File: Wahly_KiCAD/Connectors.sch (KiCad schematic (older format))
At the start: 9 parts, among them J2 Power, J3 ADC, J4 SWD, J5 TIM2

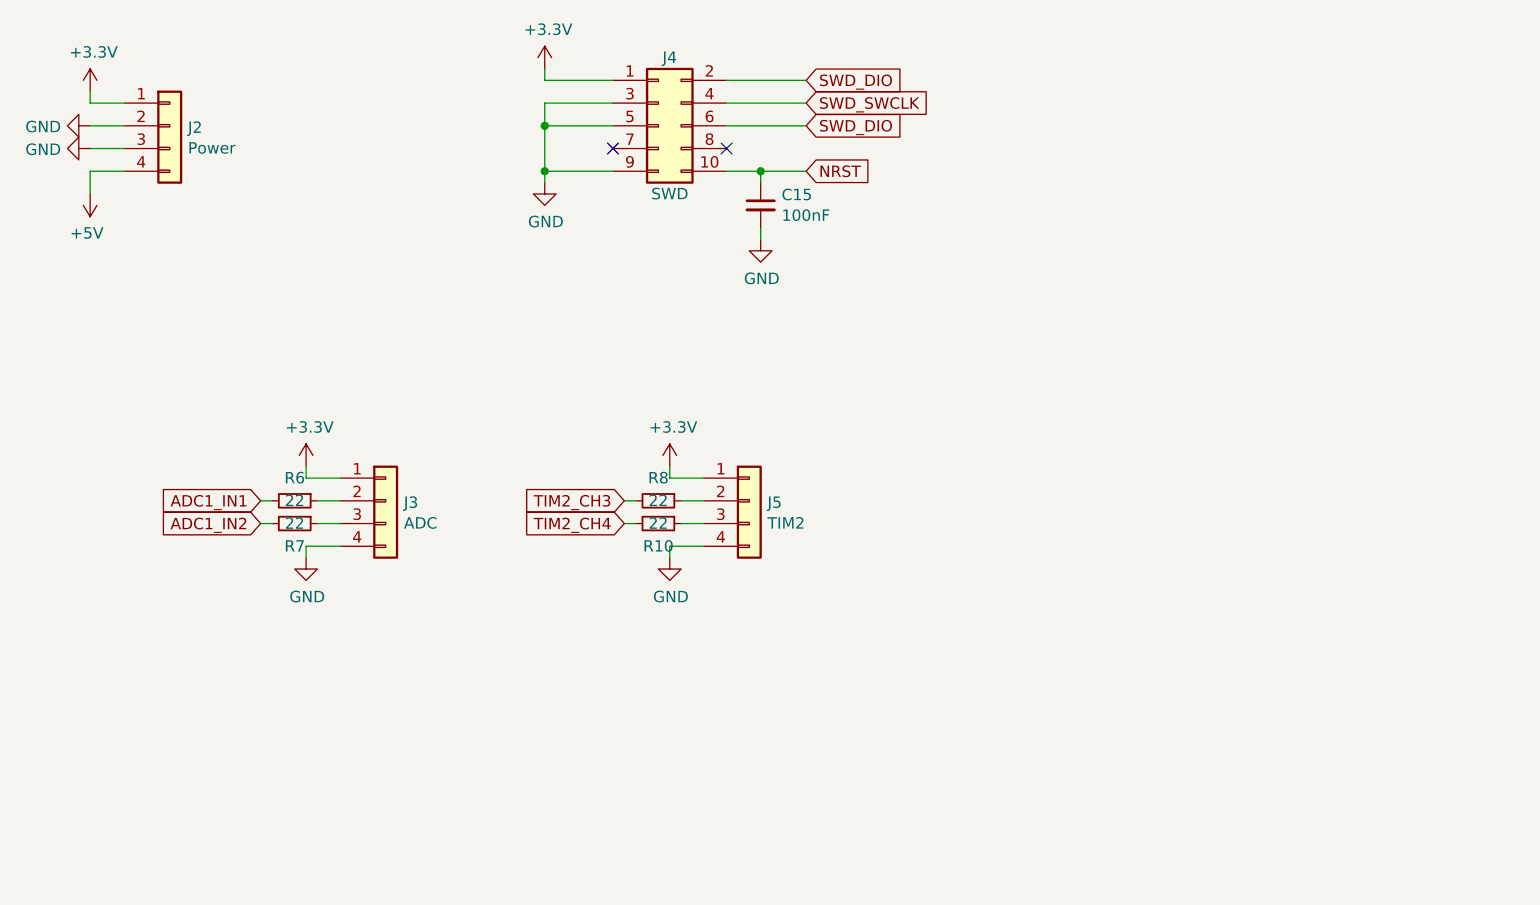
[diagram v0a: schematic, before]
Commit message: pdf schematic
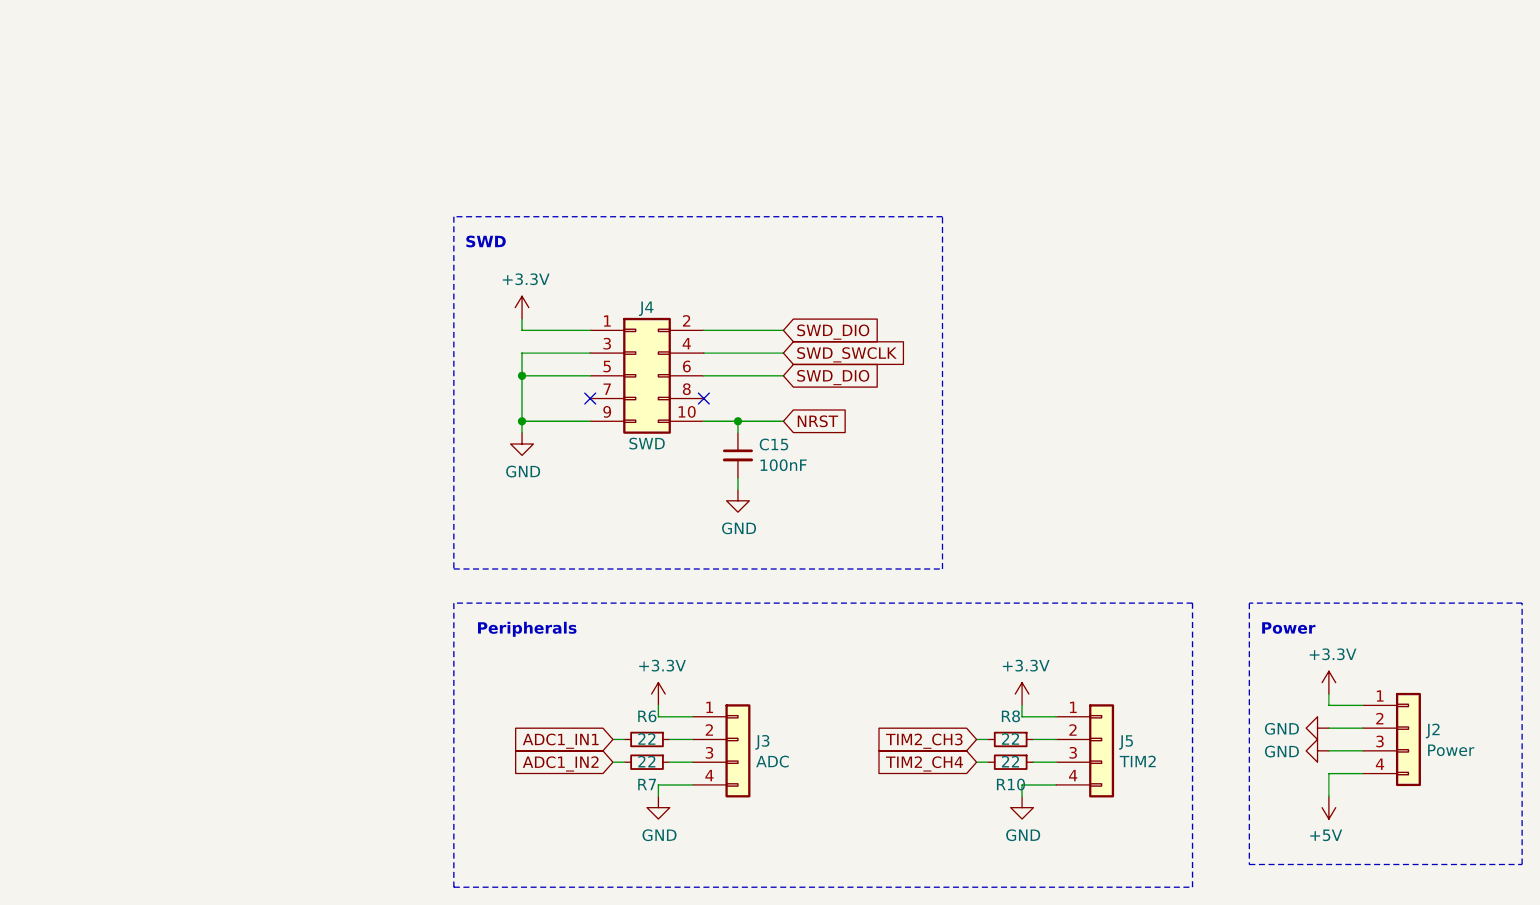
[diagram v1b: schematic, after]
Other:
- note added: "Peripherals"
- note added: "Power"
- note added: "SWD"
- moved on the sheet: C15, J2, J3, J4, J5, R10, R6, R7, R8

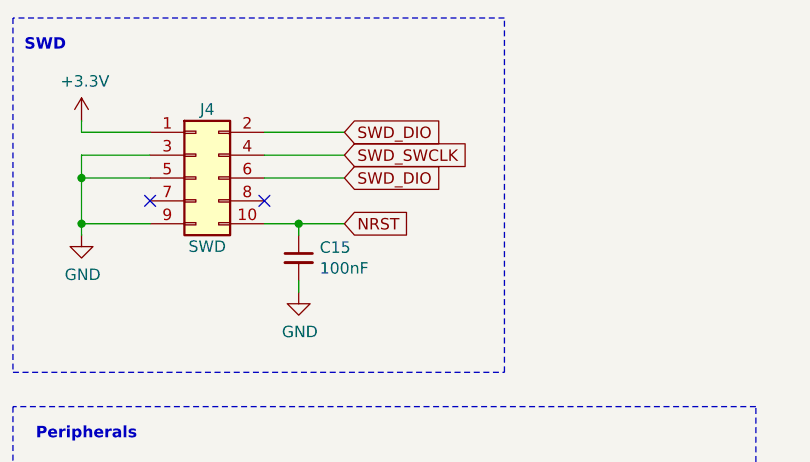
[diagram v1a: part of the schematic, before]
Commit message: Silkscreen & DRC
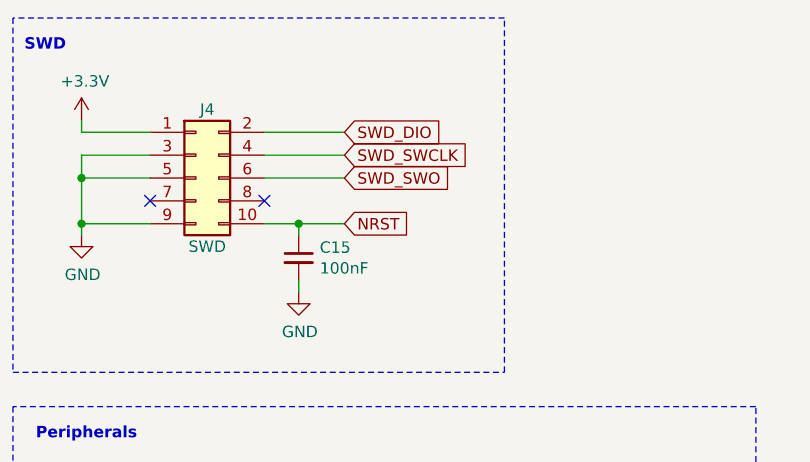
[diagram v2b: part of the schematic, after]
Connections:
- net SWD_DIO: no longer J4.6 (Pin_6)
- new net SWD_SWO: J4.6 (Pin_6)
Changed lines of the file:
@@
 NoConn ~ 4250 2600
 Text GLabel 5100 2500 2    50   Input ~ 0
-SWD_DIO
+SWD_SWO
 Wire Wire Line
 	5100 2500 4750 2500
